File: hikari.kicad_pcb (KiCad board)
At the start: 2 copper layers, 76 x 84 mm, 48 parts, among them SW1 SW_PUSH, U1 ProMicro

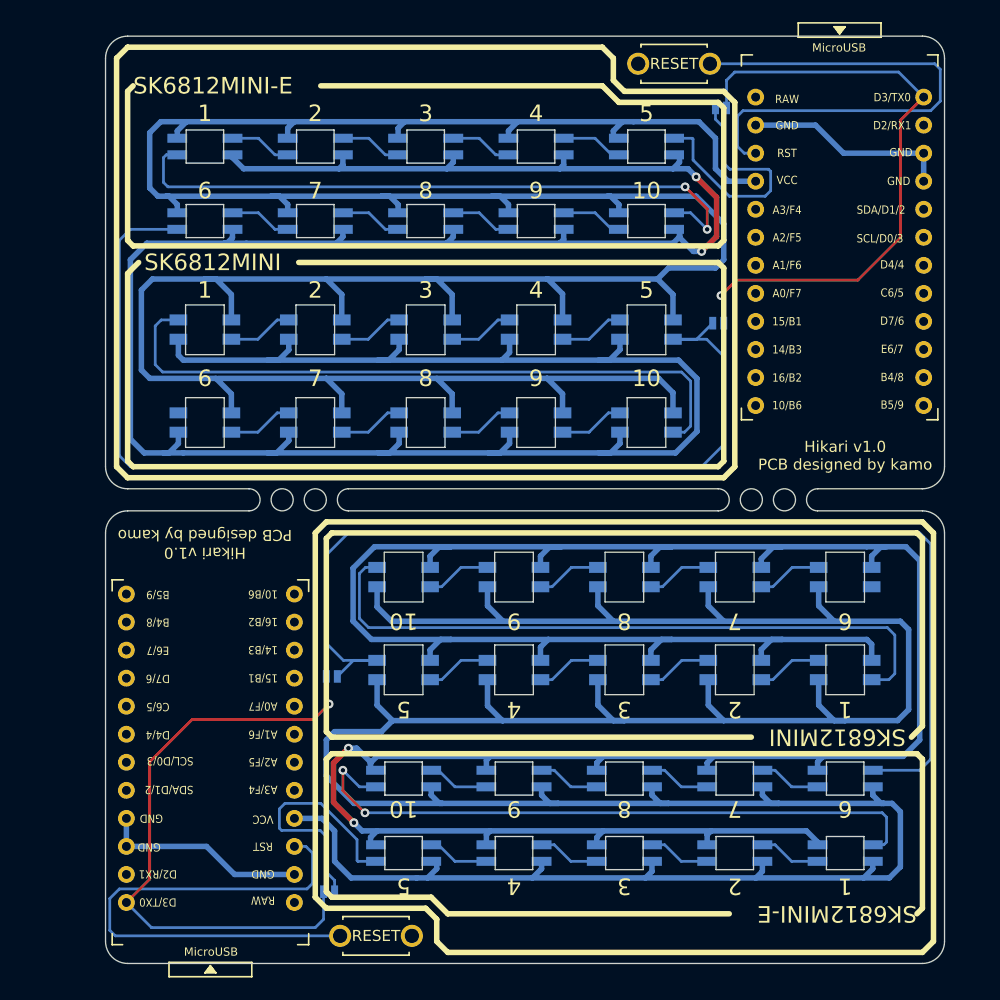
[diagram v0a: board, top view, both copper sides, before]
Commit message: :sparkles: (recreate pcb)
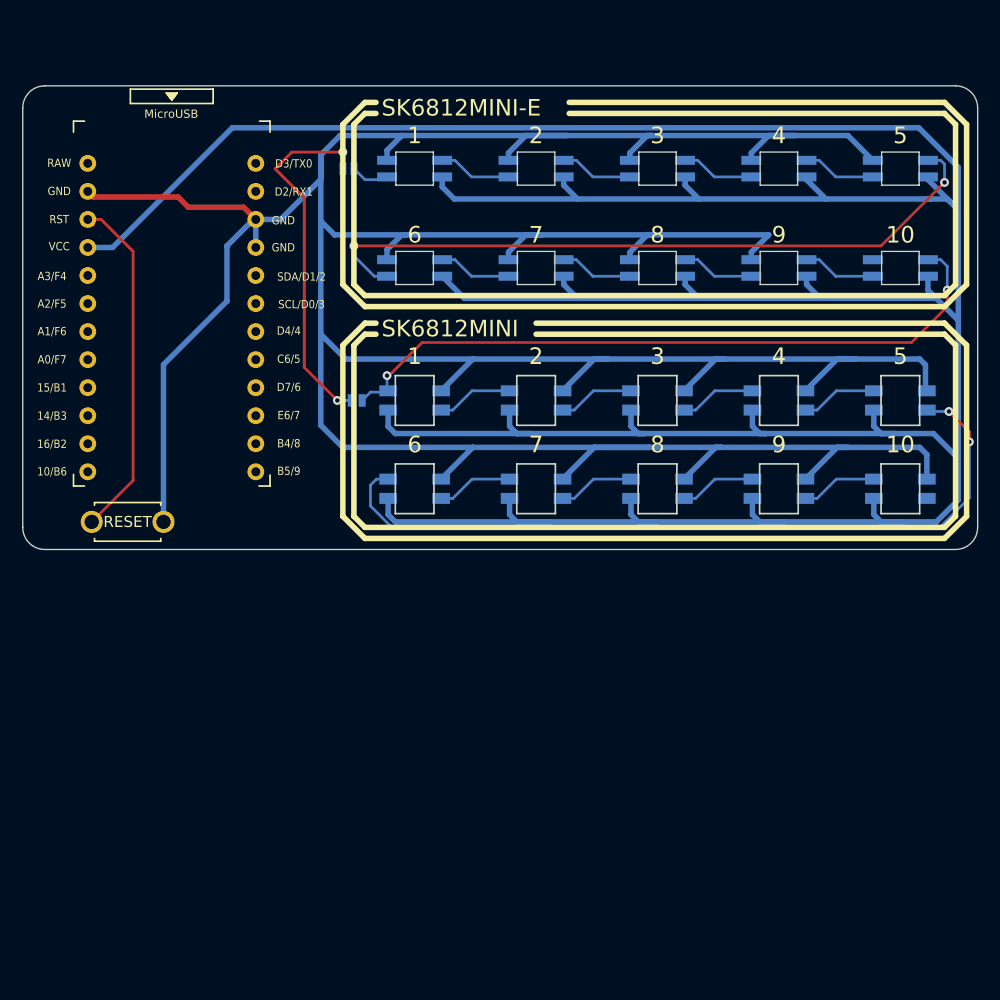
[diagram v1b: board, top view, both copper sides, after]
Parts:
- removed the JP1 at (111.2, 122.5)
- removed the JP1 at (146.8, 51.5)
- removed the JP2 at (111.5, 103.0)
- removed the JP2 at (146.5, 71.0)
- removed the L1 at (118.0, 119.0)
- removed the L1 at (140.0, 55.0)
- removed the L10 at (158.0, 112.2)
- removed the L10 at (100.0, 61.8)
- removed the L11 at (118.0, 102.4)
- removed the L11 at (140.0, 71.6)
- removed the L12 at (128.0, 102.4)
- removed the L12 at (130.0, 71.6)
- removed the L13 at (138.0, 102.4)
- removed the L13 at (120.0, 71.6)
- removed the L14 at (148.0, 102.4)
- removed the L14 at (110.0, 71.6)
- removed the L15 at (158.0, 102.4)
- removed the L15 at (100.0, 71.6)
- removed the L16 at (118.0, 94.0)
- removed the L16 at (140.0, 80.0)
- removed the L17 at (128.0, 94.0)
- removed the L17 at (130.0, 80.0)
- removed the L18 at (138.0, 94.0)
- removed the L18 at (120.0, 80.0)
- removed the L19 at (148.0, 94.0)
- removed the L19 at (110.0, 80.0)
- removed the L2 at (128.0, 119.0)
- removed the L2 at (130.0, 55.0)
- removed the L20 at (158.0, 94.0)
- removed the L20 at (100.0, 80.0)
- removed the L3 at (138.0, 119.0)
- removed the L3 at (120.0, 55.0)
- removed the L4 at (148.0, 119.0)
- removed the L4 at (110.0, 55.0)
- removed the L5 at (158.0, 119.0)
- removed the L5 at (100.0, 55.0)
- removed the L6 at (118.0, 112.2)
- removed the L6 at (140.0, 61.8)
- removed the L7 at (128.0, 112.2)
- removed the L7 at (130.0, 61.8)
- removed the L8 at (138.0, 112.2)
- removed the L8 at (120.0, 61.8)
- removed the L9 at (148.0, 112.2)
- removed the L9 at (110.0, 61.8)
- removed the SW1 at (115.5, 126.5)
- removed the SW1 at (142.5, 47.5)
- removed the U1 at (100.5, 109.0)
- removed the U1 at (157.5, 65.0)
- added JP1: JP1, swanmatch:Jumper, B.Cu at (113.0, 57.0)
- added JP2: JP2, swanmatch:Jumper, B.Cu at (113.8, 78.0)
- added L1: SK6812MINI-E, swanmatch:YS-SK6812MINI-E, B.Cu at (119.0, 57.0)
- added L10: SK6812MINI-E, swanmatch:YS-SK6812MINI-E, B.Cu at (163.0, 66.0)
- added L11: SK6812MINI, mikamo3:SK6812MINI_1side, F.Cu at (119.0, 78.0)
- added L12: SK6812MINI, mikamo3:SK6812MINI_1side, F.Cu at (130.0, 78.0)
- added L13: SK6812MINI, mikamo3:SK6812MINI_1side, F.Cu at (141.0, 78.0)
- added L14: SK6812MINI, mikamo3:SK6812MINI_1side, F.Cu at (152.0, 78.0)
- added L15: SK6812MINI, mikamo3:SK6812MINI_1side, F.Cu at (163.0, 78.0)
- added L16: SK6812MINI, mikamo3:SK6812MINI_1side, F.Cu at (119.0, 86.0)
- added L17: SK6812MINI, mikamo3:SK6812MINI_1side, F.Cu at (130.0, 86.0)
- added L18: SK6812MINI, mikamo3:SK6812MINI_1side, F.Cu at (141.0, 86.0)
- added L19: SK6812MINI, mikamo3:SK6812MINI_1side, F.Cu at (152.0, 86.0)
- added L2: SK6812MINI-E, swanmatch:YS-SK6812MINI-E, B.Cu at (130.0, 57.0)
- added L20: SK6812MINI, mikamo3:SK6812MINI_1side, F.Cu at (163.0, 86.0)
- added L3: SK6812MINI-E, swanmatch:YS-SK6812MINI-E, B.Cu at (141.0, 57.0)
- added L4: SK6812MINI-E, swanmatch:YS-SK6812MINI-E, B.Cu at (152.0, 57.0)
- added L5: SK6812MINI-E, swanmatch:YS-SK6812MINI-E, B.Cu at (163.0, 57.0)
- added L6: SK6812MINI-E, swanmatch:YS-SK6812MINI-E, B.Cu at (119.0, 66.0)
- added L7: SK6812MINI-E, swanmatch:YS-SK6812MINI-E, B.Cu at (130.0, 66.0)
- added L8: SK6812MINI-E, swanmatch:YS-SK6812MINI-E, B.Cu at (141.0, 66.0)
- added L9: SK6812MINI-E, swanmatch:YS-SK6812MINI-E, B.Cu at (152.0, 66.0)
- added SW1: SW_PUSH, swanmatch:ResetSW_1side, F.Cu at (93.0, 89.0)
- added U1: ProMicro, swanmatch:ProMicro_v3.5, F.Cu at (97.0, 71.0)
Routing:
- net (no net): track 1016.7 -> 0.00 mm, vias 5 -> 0
- net VCC: track 291.6 -> 373.0 mm
- net GND: track 286.3 -> 367.6 mm, vias 2 -> 0
- net Net-(JP2-Pad2): track 98.6 -> 63.1 mm, vias 0 -> 2
- net Net-(JP1-Pad1): track 56.2 -> 32.8 mm, vias 1 -> 2
- net Net-(JP1-Pad2): track 23.4 -> 3.52 mm
- net Net-(SW1-Pad2): track 47.5 -> 32.1 mm
- net Net-(L15-Pad1): track 60.8 -> 70.6 mm, vias 0 -> 2
- net Net-(L5-Pad2): track 58.8 -> 63.8 mm
- net Net-(L8-Pad2): track 5.62 -> 6.62 mm
- net Net-(L7-Pad2): track 5.62 -> 6.62 mm
- net Net-(L4-Pad2): track 5.62 -> 6.62 mm
- net Net-(L3-Pad2): track 5.62 -> 6.62 mm
- net Net-(L2-Pad2): track 5.62 -> 6.62 mm
- net Net-(L19-Pad1): track 5.92 -> 6.92 mm
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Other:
- board size 76 x 84 mm -> 86.5 x 42 mm
